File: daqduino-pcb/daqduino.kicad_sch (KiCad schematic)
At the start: 12 parts, among them J1 24v Power Input, J2 Conn_2Rows-07Pins, J3 Conn_02x06_Counter_Clockwise, U1 LM358, U2 L7812

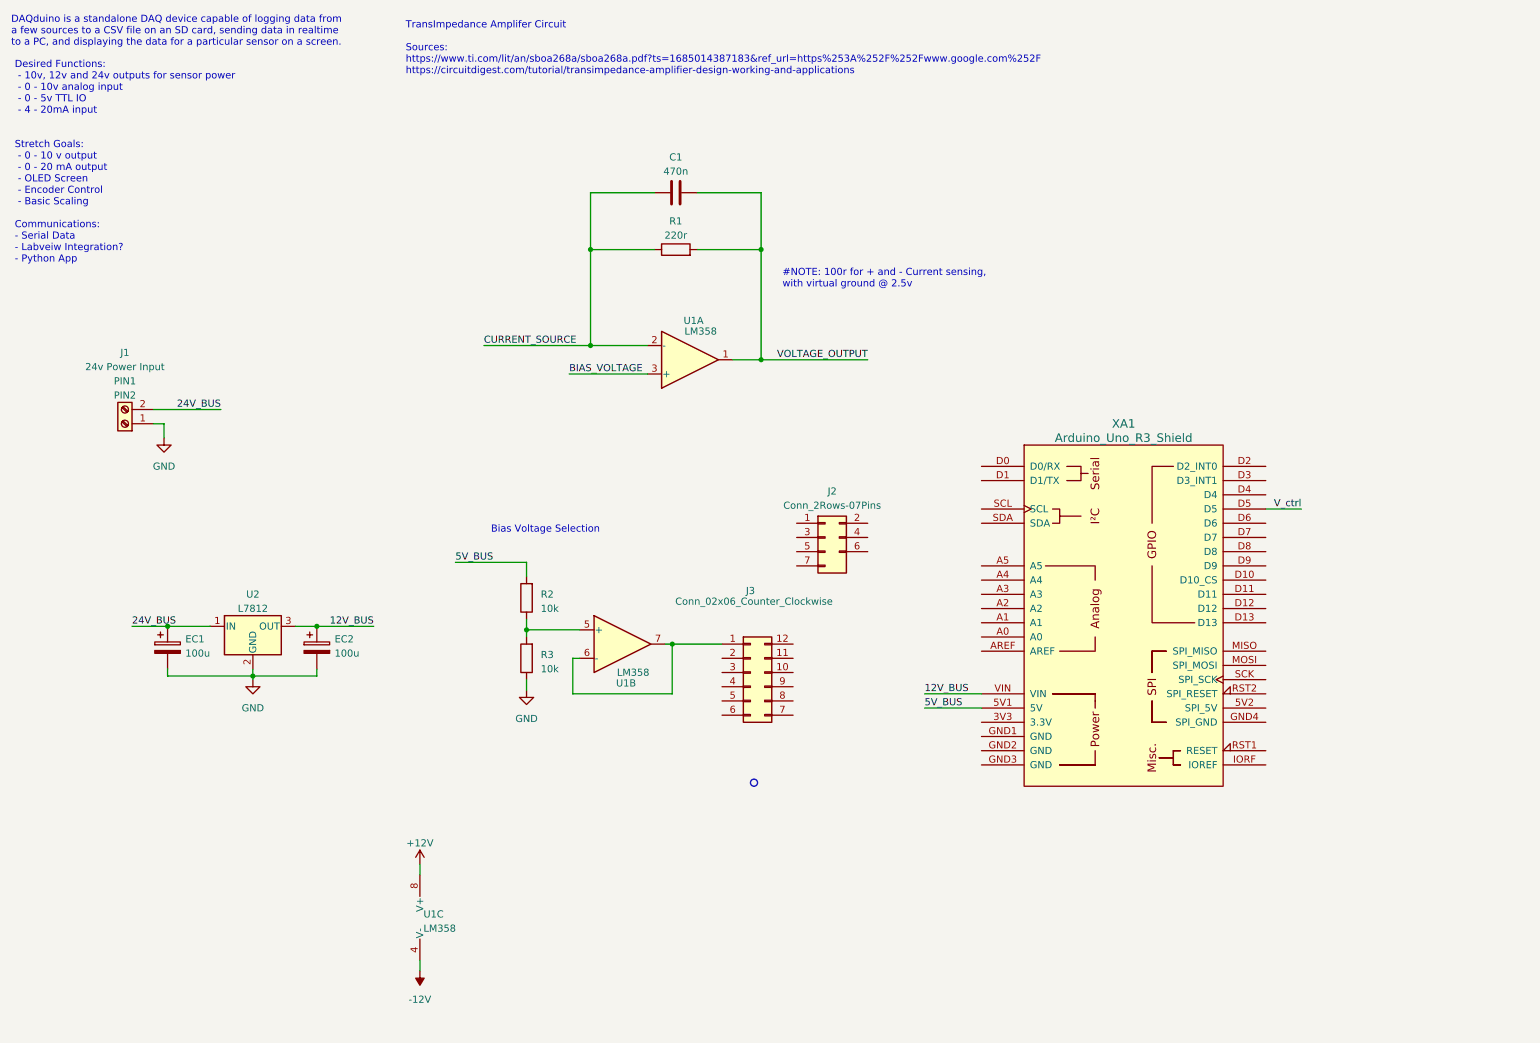
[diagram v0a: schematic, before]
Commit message: almost finished schematic
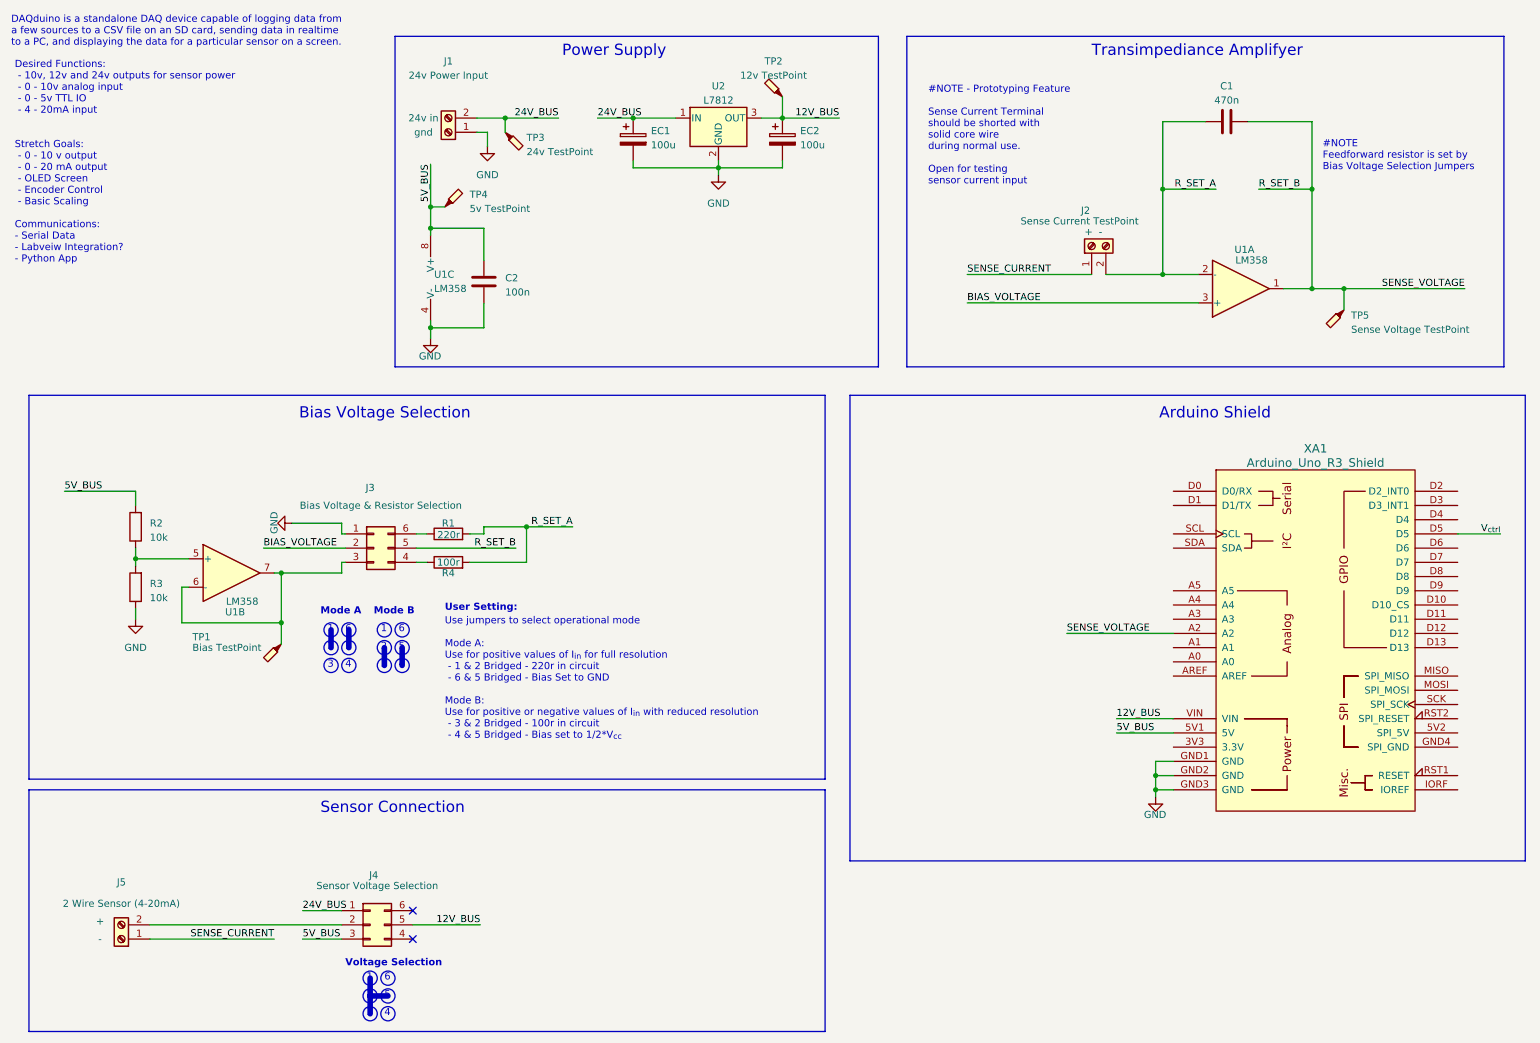
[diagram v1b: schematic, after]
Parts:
- removed J2: Conn_2Rows-07Pins, symbol Connector_Generic:Conn_2Rows-07Pins
- removed J3: Conn_02x06_Counter_Clockwise, symbol Connector_Generic:Conn_02x06_Counter_Clockwise
- added C2: 100n, 000_Capacitors_Immo:C_0805_2012_HandSolder_kawaii, symbol 000_Capacitor_Film_Immo:100n
- added J2: Sense Current TestPoint, 000 Connectors Immo:TerminalBlock_Altech_AK300-2_P5.00mm, symbol 000_Connectors_Immo:Screw_Terminal_01x02
- added J3: Bias Voltage & Resistor Selection, symbol Connector_Generic:Conn_02x03_Counter_Clockwise
- added J4: Sensor Voltage Selection, symbol Connector_Generic:Conn_02x03_Counter_Clockwise
- added J5: 2 Wire Sensor (4-20mA), 000 Connectors Immo:TerminalBlock_Altech_AK300-2_P5.00mm, symbol 000_Connectors_Immo:Screw_Terminal_01x02
- added R4: 100r, symbol Device:R
- added TP1: Bias TestPoint, TestPoint:TestPoint_Bridge_Pitch2.54mm_Drill1.0mm, symbol Connector:TestPoint_Probe
- added TP2: 12v TestPoint, TestPoint:TestPoint_Bridge_Pitch2.54mm_Drill1.0mm, symbol Connector:TestPoint_Probe
- added TP3: 24v TestPoint, TestPoint:TestPoint_Bridge_Pitch2.54mm_Drill1.0mm, symbol Connector:TestPoint_Probe
- added TP4: 5v TestPoint, TestPoint:TestPoint_Bridge_Pitch2.54mm_Drill1.0mm, symbol Connector:TestPoint_Probe
- added TP5: Sense Voltage TestPoint, TestPoint:TestPoint_Bridge_Pitch2.54mm_Drill1.0mm, symbol Connector:TestPoint_Probe
- J1: PIN1 PIN1 -> gnd; PIN2 PIN2 -> 24v in
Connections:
- net +12V is gone; now on net 5V_BUS: U1.8 (V+)
- net -12V is gone; now on net GND: U1.4 (V-)
- net 12V_BUS: now also J4.5 (Pin_5), TP2.1
- net 24V_BUS: now also J4.1 (Pin_1), TP3.1
- net 5V_BUS: now also C2.1, J4.3 (Pin_3), TP4.1
- net BIAS_VOLTAGE: now also J3.2 (Pin_2)
- net GND: now also XA1.GND1 (GND), XA1.GND2 (GND), XA1.GND3 (GND), C2.2, J3.1 (Pin_1)
- net at U1.6 (-), U1.7: now also J3.3 (Pin_3), TP1.1
- net R_SET_B: now reaches XA1.A2
- net R_SET_B: now also C1.2, U1.1, J3.5 (Pin_5), TP5.1
- net CURRENT_SOURCE renamed R_SET_A
- net R_SET_A: now also R1.2, J2.2 (Pin_2), R4.2; no longer R1.1
- removed net VOLTAGE_OUTPUT: C1.2, R1.2, U1.1
- net V_ctrl renamed V_{ctrl}
- new net: J4.2 (Pin_2), J5.2 (Pin_2)
- new net: J3.4 (Pin_4), R4.1
- new net: J3.6 (Pin_6), R1.1
- new net SENSE_CURRENT: J2.1 (Pin_1), J5.1 (Pin_1)
- no-connect marks 0 -> 2
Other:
- note added: "#NOTE - Prototyping Feature Sense Current Terminal should be shorted with solid core wire during normal use. Open for testing sensor current input"
- note added: "#NOTE Feedforward resistor is set by Bias Voltage Selection Jumpers"
- note added: "1"
- note added: "2"
- note added: "3"
- note added: "4"
- note added: "5"
- note added: "6"
- note added: "Arduino Shield"
- note added: "Mode A"
- note added: "Mode B"
- note added: "Power Supply"
- note added: "Sensor Connection"
- note added: "Transimpediance Amplifyer"
- note added: "Use jumpers to select operational mode Mode A: Use for positive values of I_{in} for full resolution - 1 & 2 Bridged - 220r in circuit - 6 & 5 Bridged - Bias Set to GND Mode B: Use for positive or negative values of I_{in} with reduced resolution - 3 & 2 Bridged - 100r in circuit - 4 & 5 Bridged - Bias set to 1/2*V_{cc}"
- note added: "User Setting:"
- note added: "Voltage Selection"
- note removed: "#NOTE: 100r for + and - Current sensing, with virtual ground @ 2.5v"
- note removed: "TransImpedance Amplifer Circuit Sources: https://www.ti.com/lit/an/sboa268a/sboa268a.pdf?ts=1685014387183&ref_url=https%253A%252F%252Fwww.google.com%252F https://circuitdigest.com/tutorial/transimpedance-amplifier-design-working-and-applications"
- moved on the sheet: C1, EC1, EC2, J1, R2, R3, U1A, U1B, U1C, U2, XA1
